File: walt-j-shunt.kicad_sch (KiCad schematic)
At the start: 13 parts, among them J1 Screw_Terminal_01x03

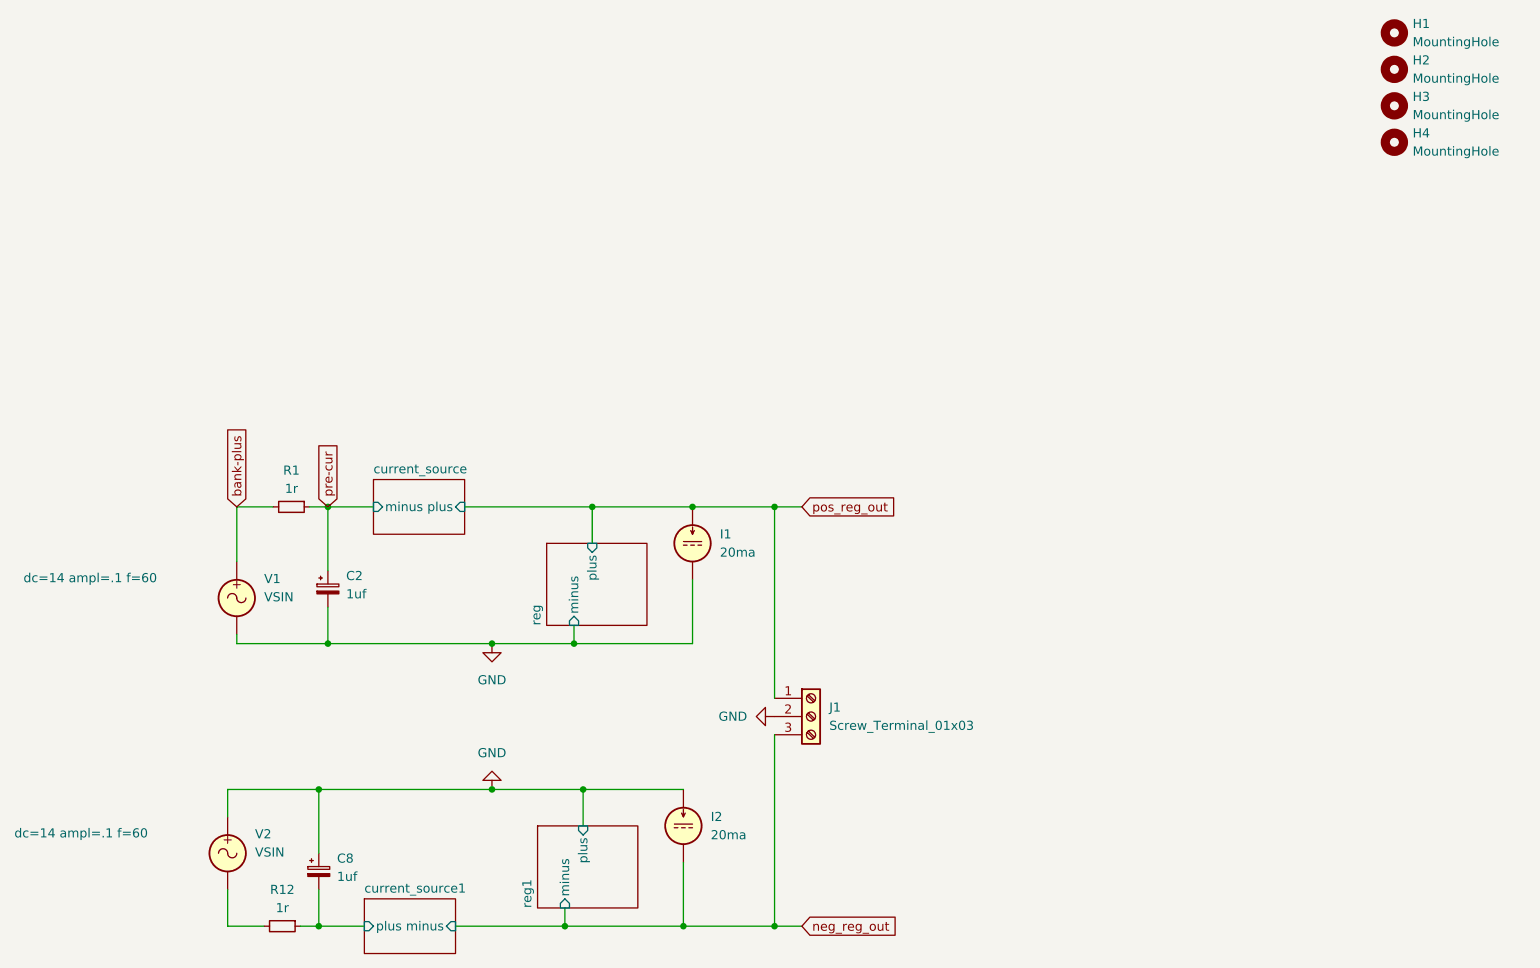
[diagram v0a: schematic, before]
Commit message: Single rail design - initial branch
🤖 Generated with [Claude Code](https://claude.ai/code)

Co-Authored-By: Claude <noreply@anthropic.com>
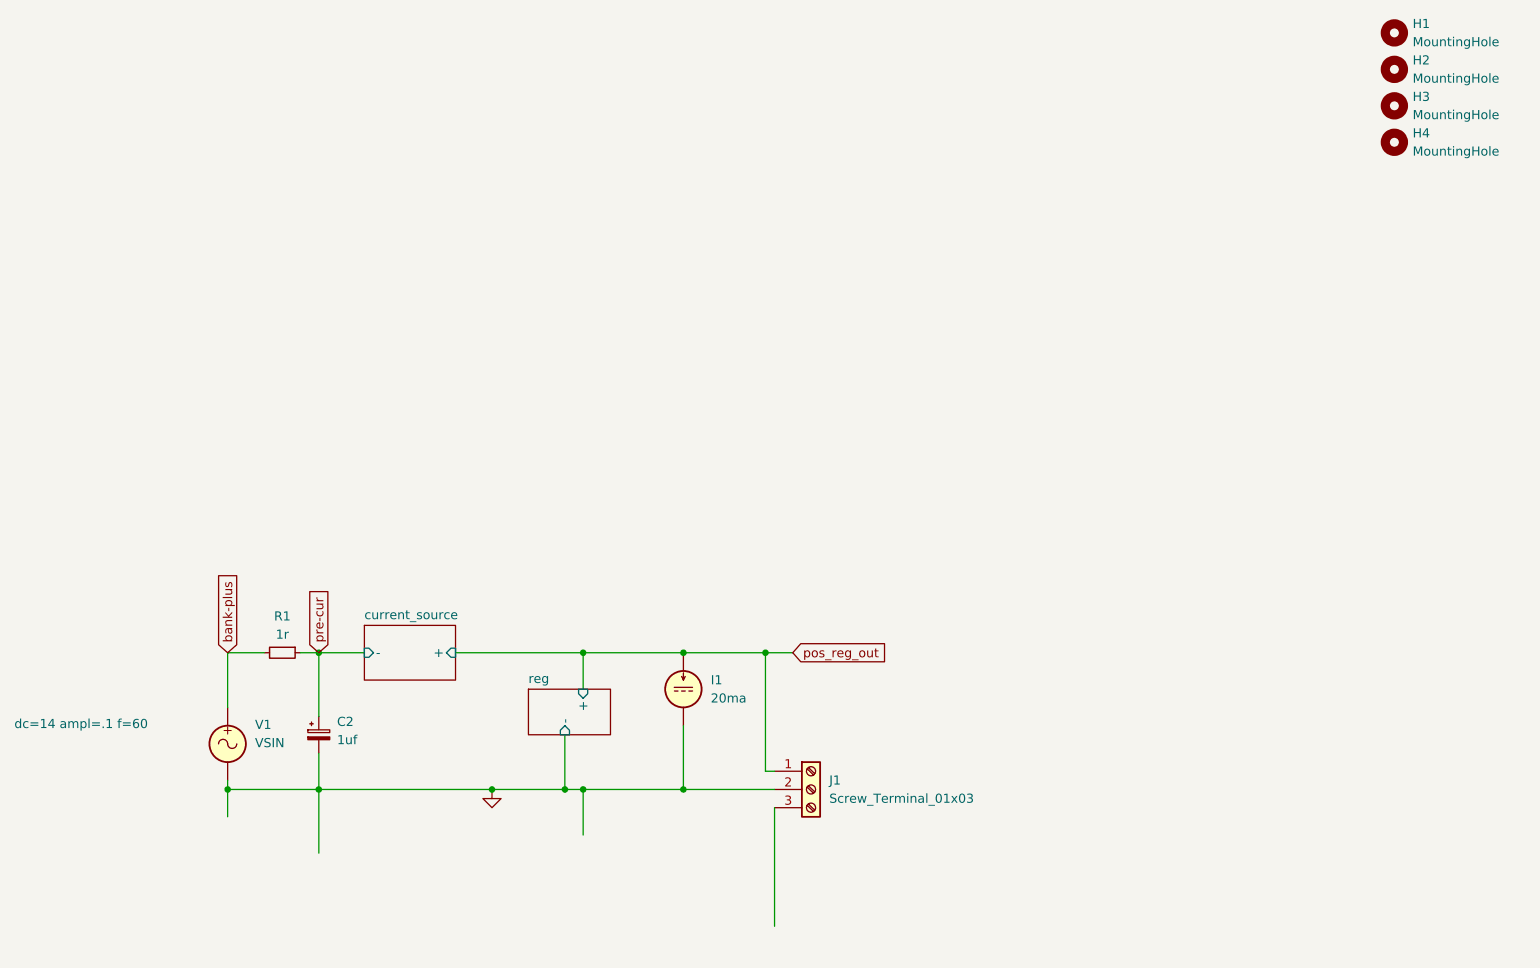
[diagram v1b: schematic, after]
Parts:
- removed C8: 1uf, Samacsys:B32529C105J, symbol Device:C_Polarized_Small
- removed I2: 20ma, Samacsys:395443002, symbol Simulation_SPICE:IDC
- removed R12: 1r, Resistor_SMD:R_0805_2012Metric, symbol Device:R_Small
- removed V2: VSIN, Connector_Molex:Molex_KK-254_AE-6410-02A_1x02_P2.54mm_Vertical, symbol Simulation_SPICE:VSIN
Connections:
- net neg_reg_out: no longer names the net of J1.3 (Pin_3)
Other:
- removed sheet current_source1
- removed sheet reg1
- sheet current_source ports: added +, -; removed minus, plus
- sheet reg ports: added +, -; removed minus, plus
- moved on the sheet: C2, I1, J1, R1, V1
